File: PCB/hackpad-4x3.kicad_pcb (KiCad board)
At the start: 2 copper layers, 89.7 x 84.5 mm, 37 parts, among them SW1 SW_Push, SW10 SW_Push, SW11 SW_Push, SW12 SW_Push, SW13 RotaryEncoder_Switch, SW2 SW_Push, SW3 SW_Push, SW4 SW_Push, SW5 SW_Push, SW6 SW_Push, SW7 SW_Push, SW8 SW_Push, SW9 SW_Push, U1 XIAO-RP2040-DIP

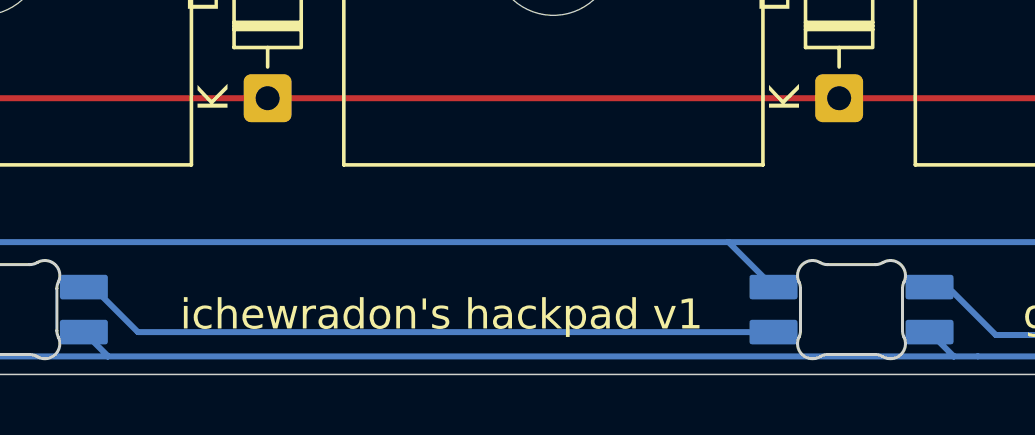
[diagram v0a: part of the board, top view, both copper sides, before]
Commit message: Update hackpad-4x3.kicad_pcb
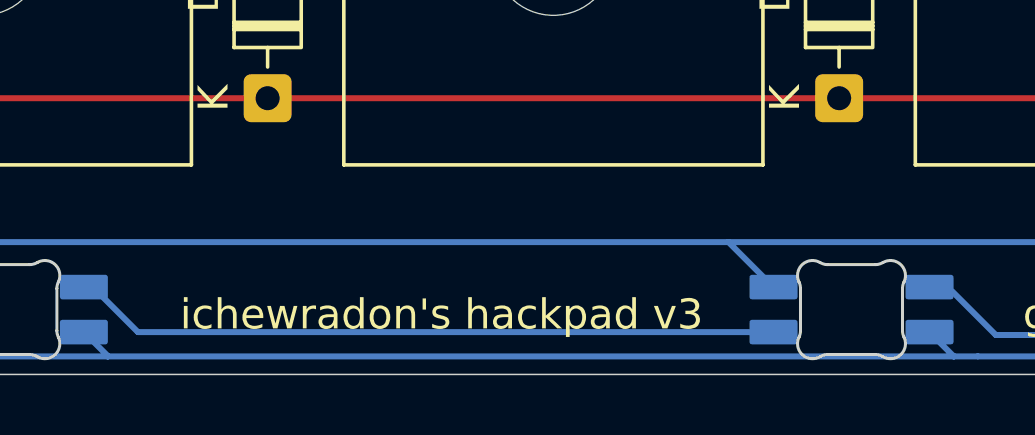
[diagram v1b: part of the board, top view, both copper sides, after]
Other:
- board text added: "ichewradon's hackpad v3"
- board text removed: "ichewradon's hackpad v1"
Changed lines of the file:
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@@
 		)
 	)
-	(gr_text "ichewradon's hackpad v1\n"
+	(gr_text "ichewradon's hackpad v3"
 		(at 120.904 114 0)
 		(layer "F.SilkS")
@@
 			(justify left bottom)
 		)
-		(render_cache "ichewradon's hackpad v1\n" 0
+		(render_cache "ichewradon's hackpad v3" 0
 			(polygon
 				(pts

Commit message: Update hackpad-4x3.kicad_pcb
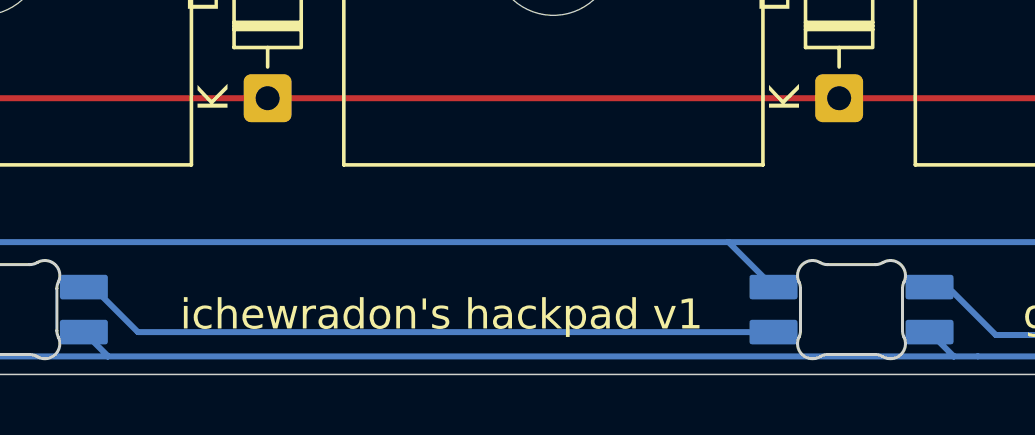
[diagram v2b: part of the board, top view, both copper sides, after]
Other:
- board text added: "ichewradon's hackpad v1"
- board text removed: "ichewradon's hackpad v3"
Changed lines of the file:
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@@
 		)
 	)
-	(gr_text "ichewradon's hackpad v3"
+	(gr_text "ichewradon's hackpad v1"
 		(at 120.904 114 0)
 		(layer "F.SilkS")
@@
 			(justify left bottom)
 		)
-		(render_cache "ichewradon's hackpad v3" 0
+		(render_cache "ichewradon's hackpad v1" 0
 			(polygon
 				(pts
